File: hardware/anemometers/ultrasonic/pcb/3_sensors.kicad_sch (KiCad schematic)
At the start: 17 parts, among them U10 APDS-9250, U11 AS3935, U8 BME280, U9 BMX160

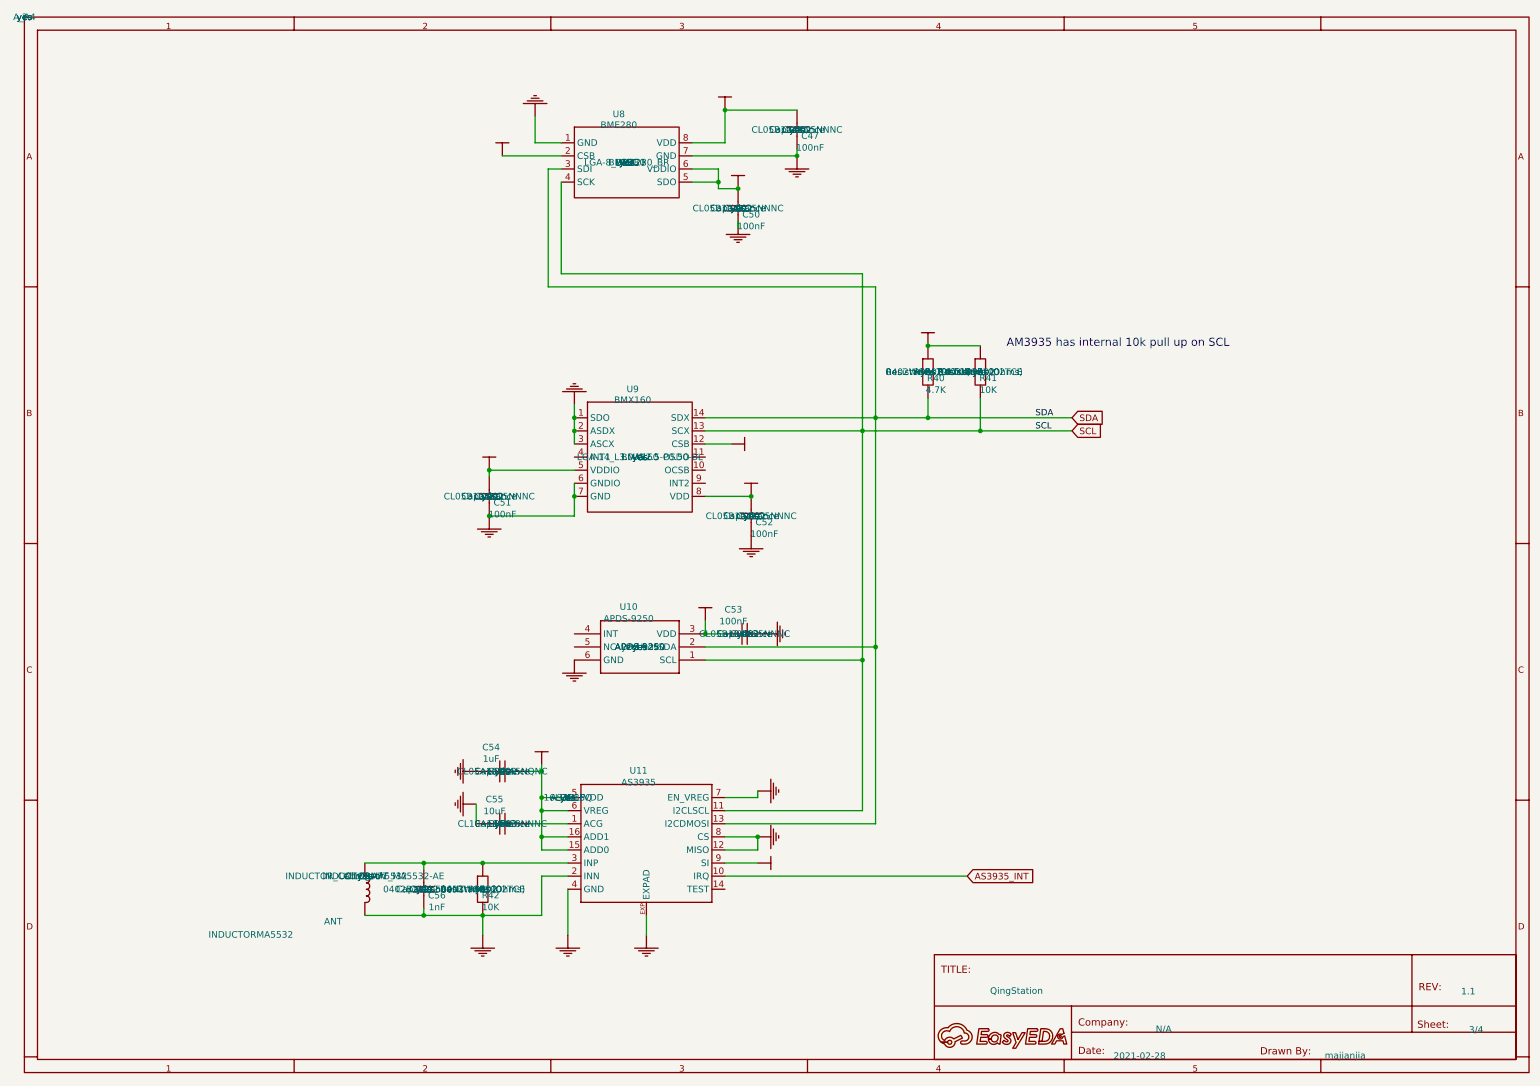
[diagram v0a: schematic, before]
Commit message: DRC clear
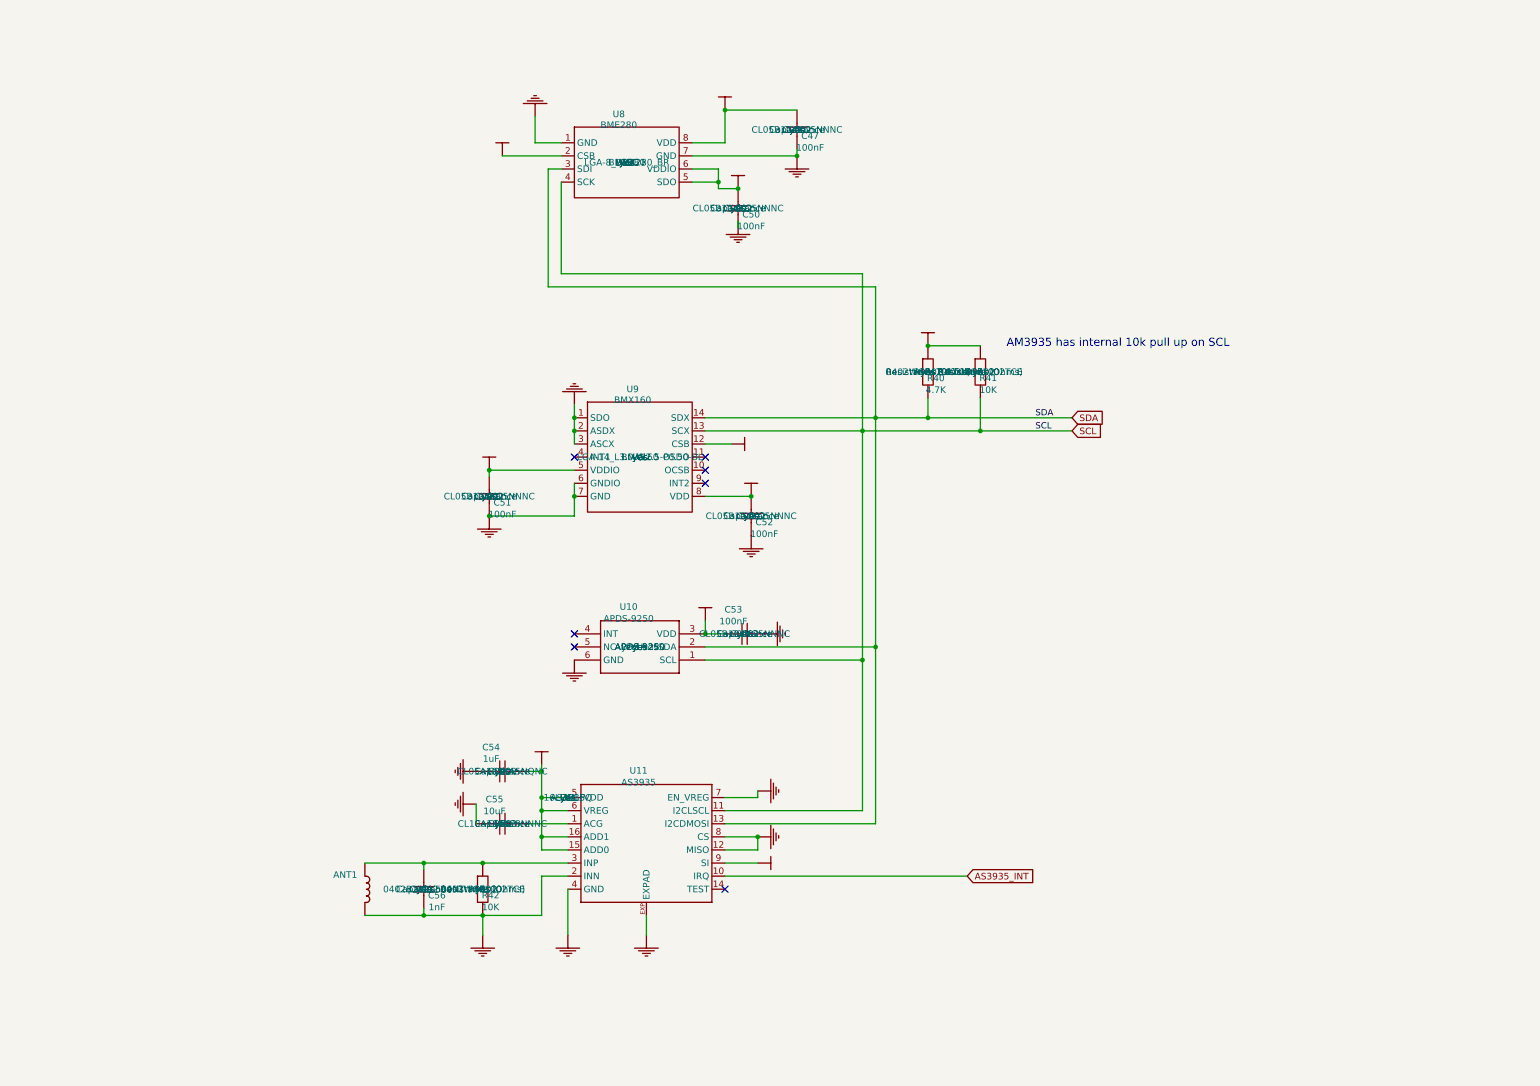
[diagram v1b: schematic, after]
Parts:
- removed ?: A_A4, ProDoc_Qin-easyedapro:, symbol ProDoc_Qin-easyedapro:A_A4
- renumbered ANT to ANT1
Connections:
- no-connect marks 0 -> 7
